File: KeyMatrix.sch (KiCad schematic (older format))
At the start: 100 parts, among them SW10 CherryMX, SW11 CherryMX, SW12 CherryMX, SW13 CherryMX, SW14 CherryMX, SW15 CherryMX, SW16 CherryMX, SW17 CherryMX, SW18 CherryMX, SW19 CherryMX, SW2 CherryMX, SW20 CherryMX, SW21 CherryMX, SW22 CherryMX, SW23 CherryMX, SW24 CherryMX, SW25 CherryMX, SW26 CherryMX, SW27 CherryMX, SW28 CherryMX, SW29 CherryMX, SW3 CherryMX, SW30 CherryMX, SW31 CherryMX, SW32 CherryMX, SW33 CherryMX, SW34 CherryMX, SW35 CherryMX, SW36 CherryMX, SW37 CherryMX, SW38 CherryMX, SW39 CherryMX, SW4 CherryMX, SW40 CherryMX, SW41 CherryMX, SW42 CherryMX, SW43 CherryMX, SW44 CherryMX, SW45 CherryMX, SW46 CherryMX, SW47 CherryMX, SW48 CherryMX, SW49 CherryMX, SW5 CherryMX, SW50 CherryMX, SW51 CherryMX, SW6 CherryMX, SW7 CherryMX, SW8 CherryMX, SW9 CherryMX

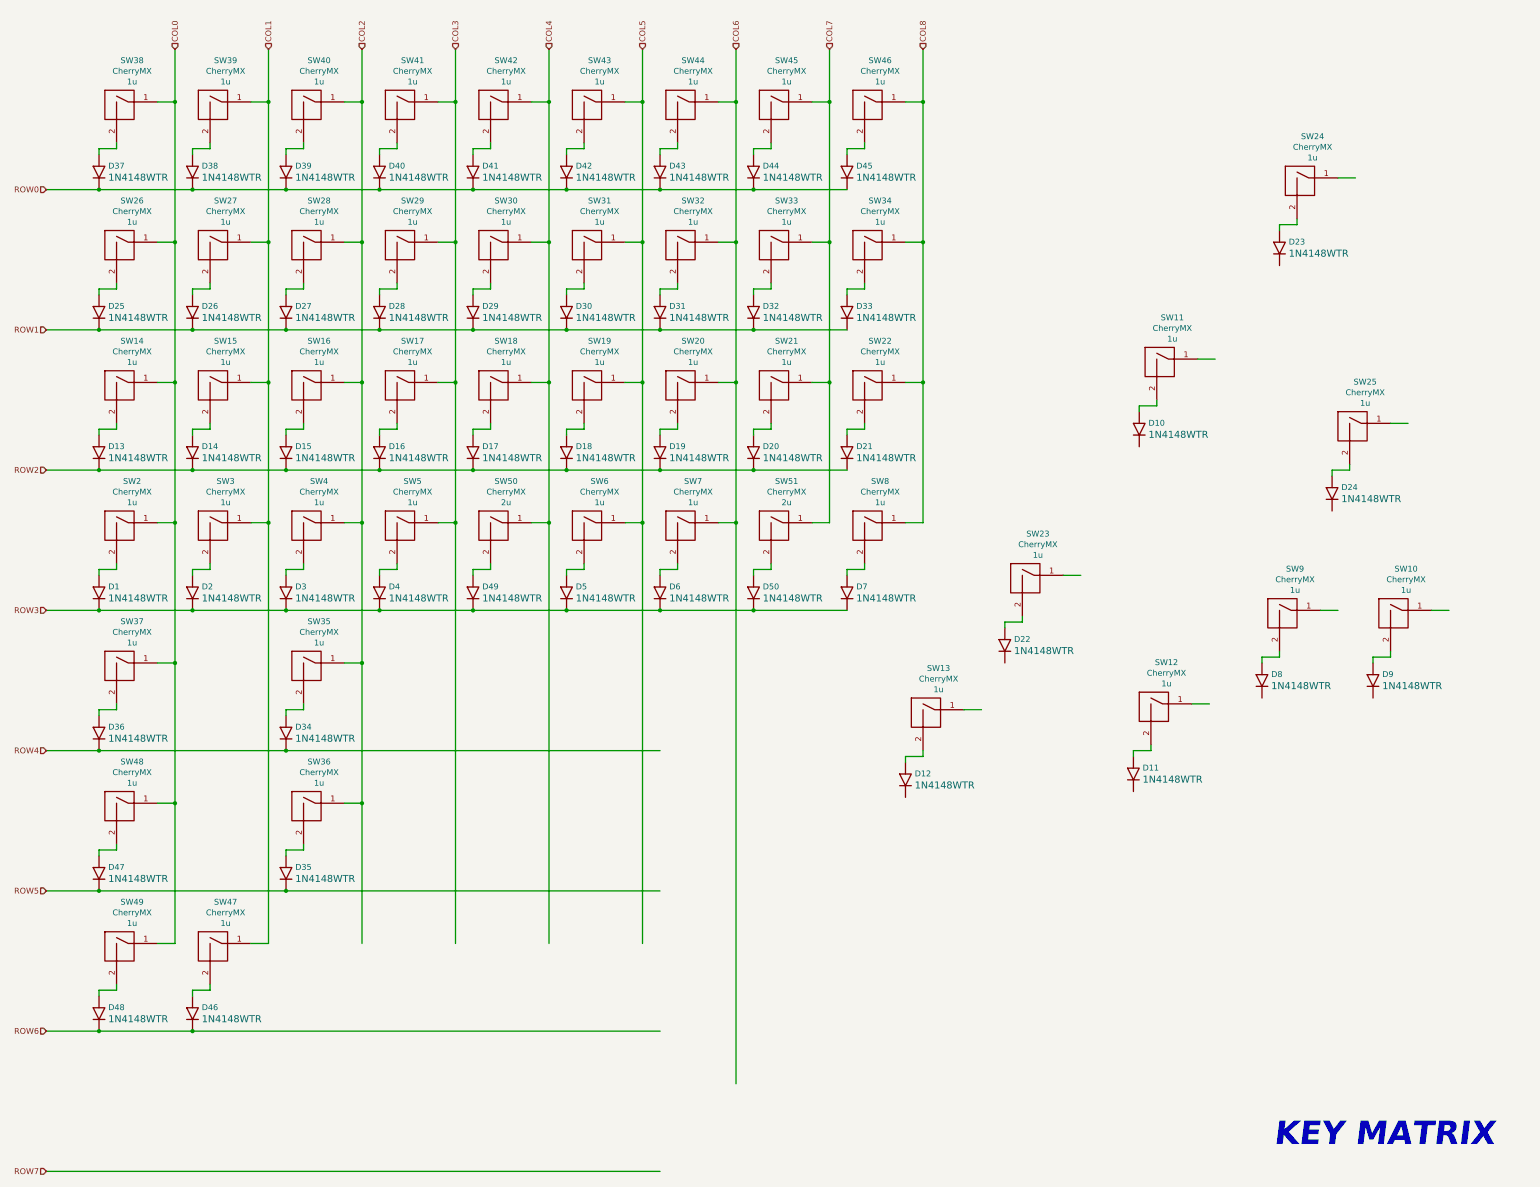
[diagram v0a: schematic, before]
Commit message: More Routing
more routing
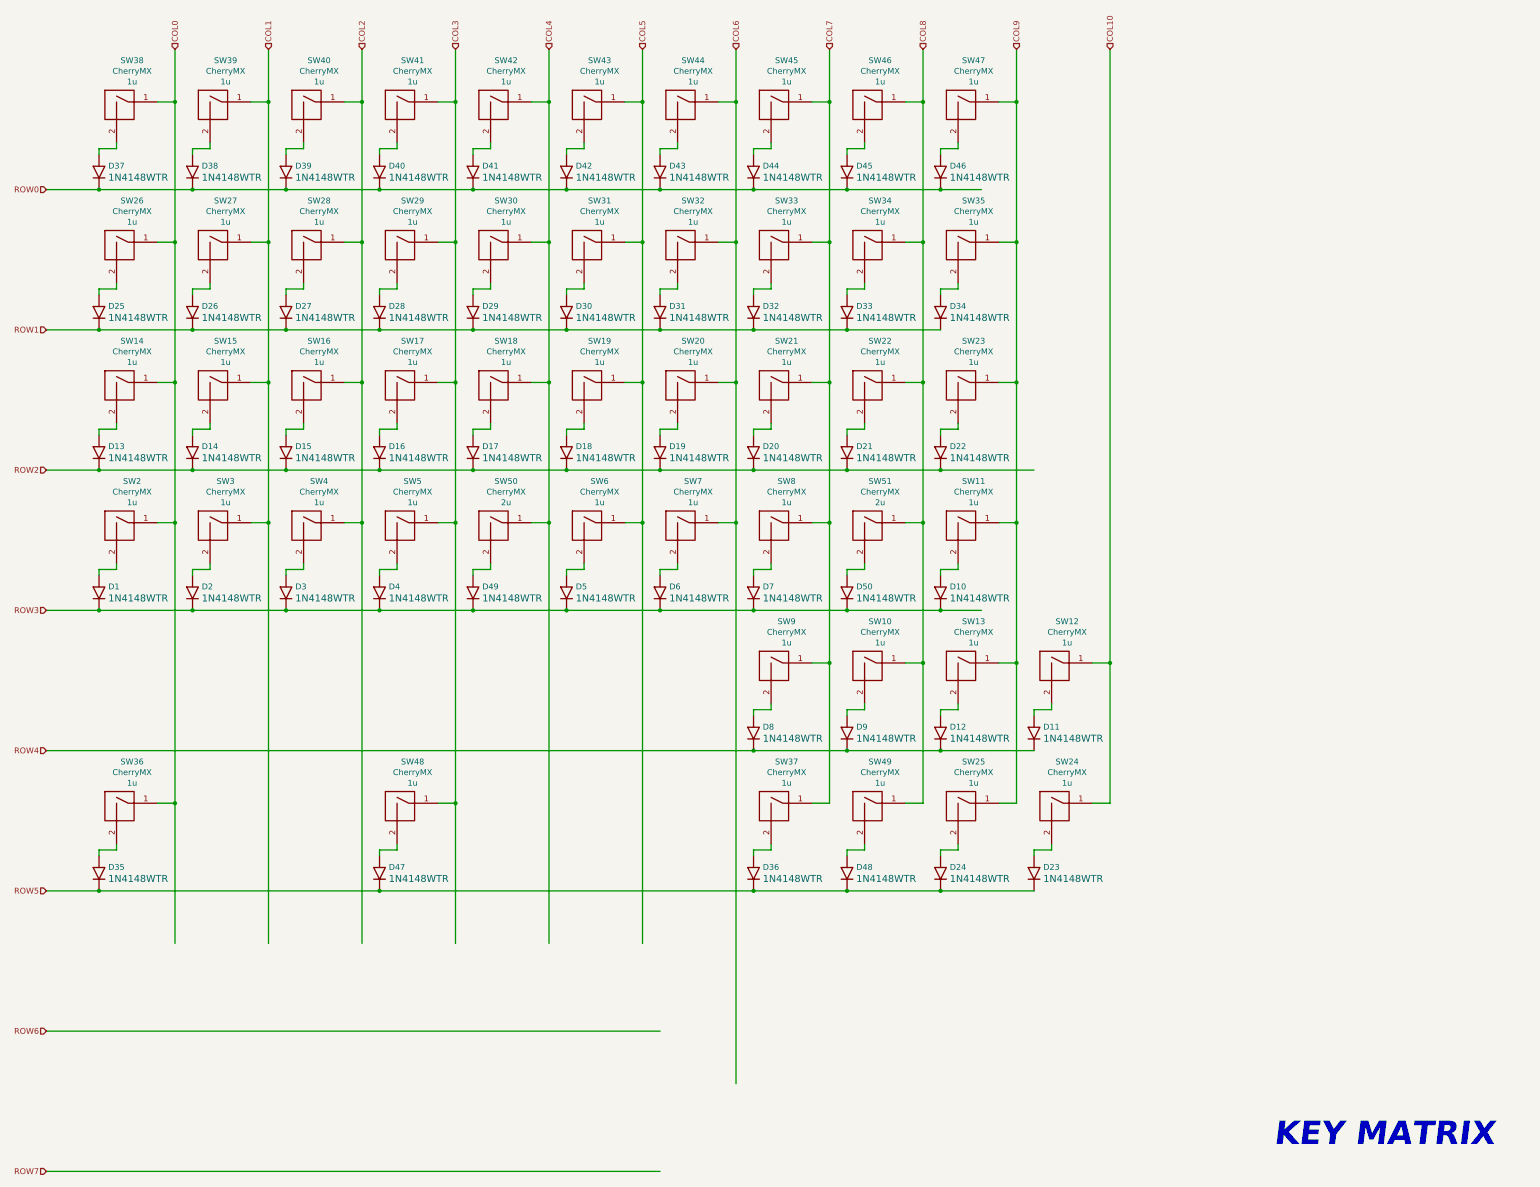
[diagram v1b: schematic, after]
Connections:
- net labels added: COL10, COL9
- wire segments 293 -> 312
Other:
- moved on the sheet: D10, D11, D12, D22, D23, D24, D34, D35, D36, D46, D47, D48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

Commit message: more routing
more routing
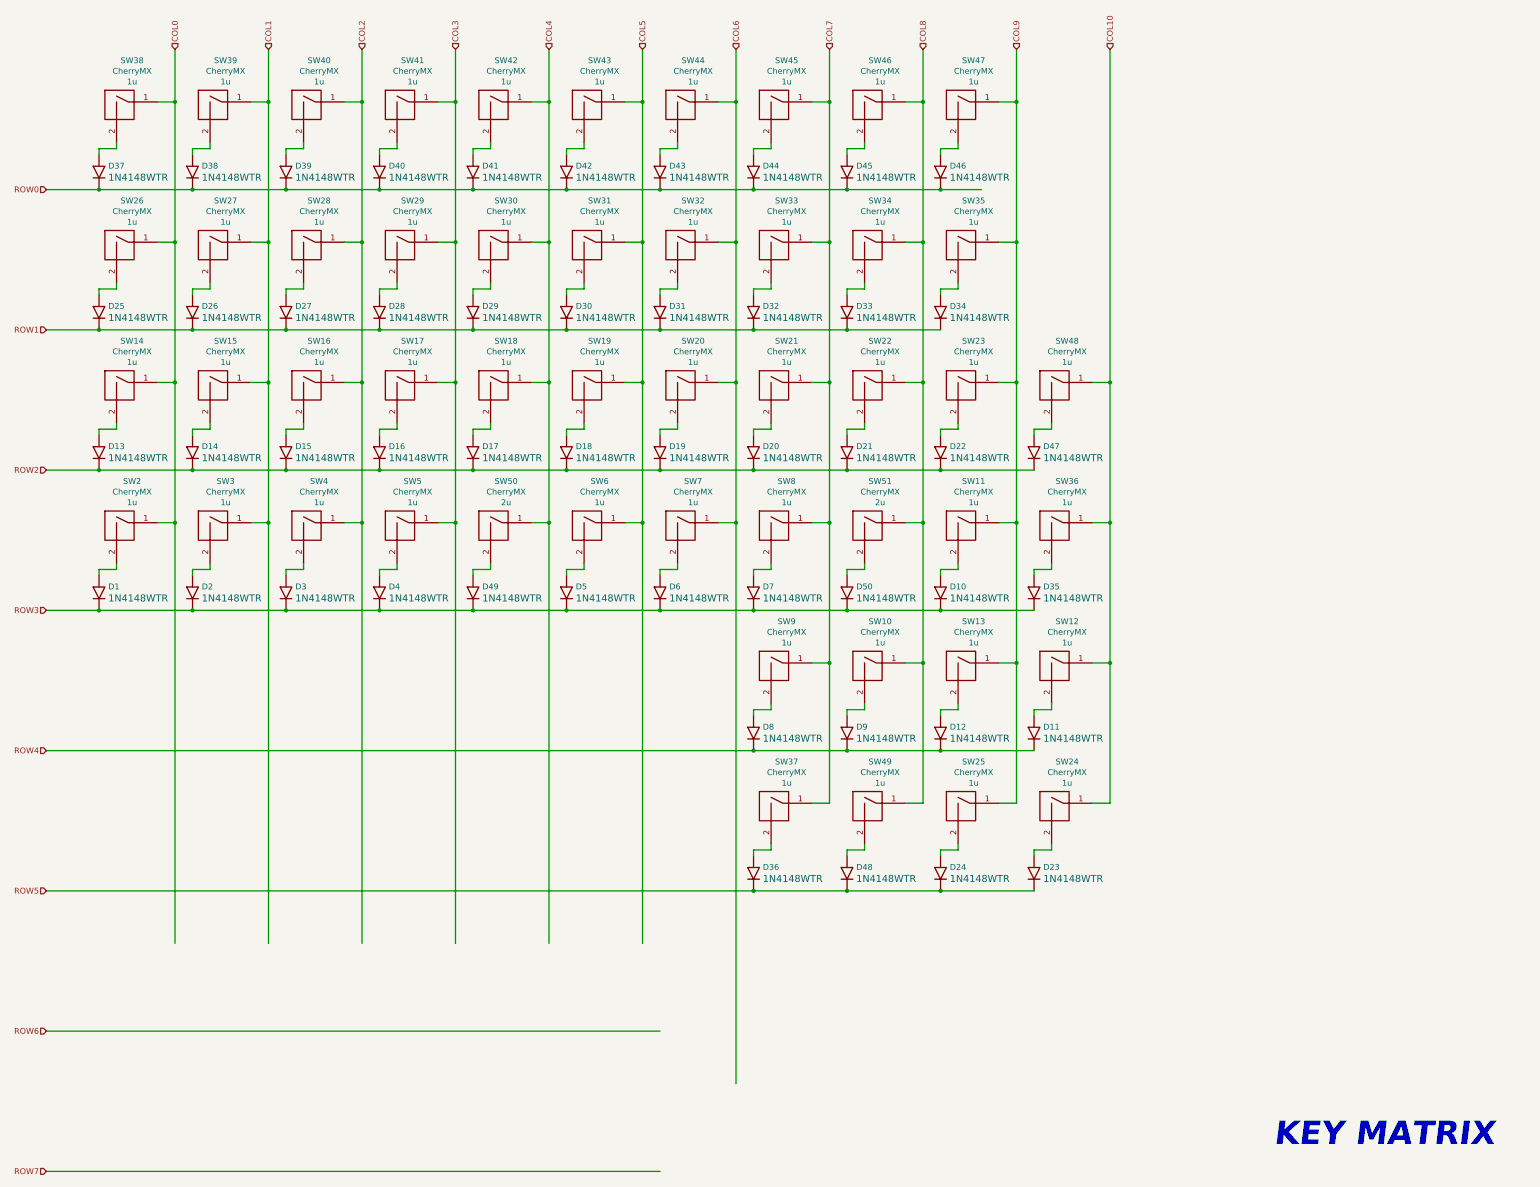
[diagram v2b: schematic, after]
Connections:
- wire segments 312 -> 310
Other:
- moved on the sheet: D35, D47, SW36, SW48
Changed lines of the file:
@@
 L MKB_Switches:CherryMX SW36
 U 1 1 5F4FA06B
-P 3000 7500
-F 0 "SW36" H 3133 7905 50  0000 C CNN
-F 1 "CherryMX" H 3133 7814 50  0000 C CNN
-F 2 "CherryMX:SW_Cherry-MX_1U_PCB-Mount_Kailh-Hot-Swap" H 3900 7600 50  0001 C CNN
-F 3 "" H 3800 7600 50  0001 C CNN
-F 4 "DNP" H 3000 7500 50  0001 C CNN "Manufacturer"
-F 5 "DNP" H 3000 7500 50  0001 C CNN "MPN"
-F 6 "DNP" H 3000 7500 50  0001 C CNN "Supplier"
-F 7 "DNP" H 3000 7500 50  0001 C CNN "Supplier PN"
-F 8 "1u" H 3133 7723 50  0000 C CNN "Package"
-	1    3000 7500
-	1    0    0    -1
-$EndComp
-Wire Wire Line
-	3500 7450 3350 7450
-Wire Wire Line
-	3000 7800 3000 7850
-Wire Wire Line
-	3000 7850 2850 7850
-Wire Wire Line
-	2850 7850 2850 7900
+P 11000 5100
+F 0 "SW36" H 11133 5505 50  0000 C CNN
+F 1 "CherryMX" H 11133 5414 50  0000 C CNN
+F 2 "CherryMX:SW_Cherry-MX_1U_PCB-Mount_Kailh-Hot-Swap" H 11900 5200 50  0001 C CNN
+F 3 "" H 11800 5200 50  0001 C CNN
+F 4 "DNP" H 11000 5100 50  0001 C CNN "Manufacturer"
+F 5 "DNP" H 11000 5100 50  0001 C CNN "MPN"
+F 6 "DNP" H 11000 5100 50  0001 C CNN "Supplier"
+F 7 "DNP" H 11000 5100 50  0001 C CNN "Supplier PN"
+F 8 "1u" H 11133 5323 50  0000 C CNN "Package"
+	1    11000 5100
+	1    0    0    -1
+$EndComp
+Wire Wire Line
+	11500 5050 11350 5050
+Wire Wire Line
+	11000 5400 11000 5450
+Wire Wire Line
+	11000 5450 10850 5450
+Wire Wire Line
+	10850 5450 10850 5500
 $Comp
 L master-vampire_General:D D35
 U 1 1 5F4FA080
-P 2850 8050
-F 0 "D35" V 2903 7971 50  0000 R CNN
-F 1 "D" H 3300 8250 50  0001 C CNN
-F 2 "ortho-40percent:SOD-123" H 2750 8050 50  0001 C CNN
-F 3 "" H 2850 8150 50  0001 C CNN
-F 4 "1N4148WTR" V 2804 7971 60  0000 R CNN "MPN"
-F 5 "SMC Diode Solutions" H 3300 8350 60  0001 C CNN "Manufacturer"
-F 6 "DigiKey" H 3150 8450 50  0001 C CNN "Supplier"
-F 7 "1655-1360-1-ND" H 3250 8550 50  0001 C CNN "Supplier PN"
-F 8 "75V" V 2850 7971 50  0001 R CNN "Voltage Rating"
-F 9 "250mA" V 2759 7971 50  0001 R CNN "Current Rating"
-F 10 "SOD-123" H 3550 8850 50  0001 C CNN "Package"
-	1    2850 8050
+P 10850 5650
+F 0 "D35" V 10903 5571 50  0000 R CNN
+F 1 "D" H 11300 5850 50  0001 C CNN
+F 2 "ortho-40percent:SOD-123" H 10750 5650 50  0001 C CNN
+F 3 "" H 10850 5750 50  0001 C CNN
+F 4 "1N4148WTR" V 10804 5571 60  0000 R CNN "MPN"
+F 5 "SMC Diode Solutions" H 11300 5950 60  0001 C CNN "Manufacturer"
+F 6 "DigiKey" H 11150 6050 50  0001 C CNN "Supplier"
+F 7 "1655-1360-1-ND" H 11250 6150 50  0001 C CNN "Supplier PN"
+F 8 "75V" V 10850 5571 50  0001 R CNN "Voltage Rating"
+F 9 "250mA" V 10759 5571 50  0001 R CNN "Current Rating"
+F 10 "SOD-123" H 11550 6450 50  0001 C CNN "Package"
+	1    10850 5650
 	0    -1   -1   0
 $EndComp
@@
 	6050 5800 6850 5800
 Connection ~ 6700 5050
-Wire Wire Line
-	2400 8200 2850 8200
-Connection ~ 2850 8200
-Connection ~ 3500 7450
-Wire Wire Line
-	3500 7450 3500 8650
 Connection ~ 9250 7000
 Connection ~ 8450 7000
 Wire Wire Line
 	8450 7000 9250 7000
-Wire Wire Line
-	3500 5050 3500 7450
 Wire Wire Line
 	9100 3850 9100 5050
@@
 Connection ~ 9900 6250
 Wire Wire Line
-	10050 5800 10400 5800
-Wire Wire Line
-	5250 8200 8450 8200
-Wire Wire Line
-	5900 5050 5900 7450
-Wire Wire Line
-	5900 7450 5900 8650
-Connection ~ 5900 7450
-Connection ~ 5250 8200
-Wire Wire Line
-	11500 1000 11500 6250
+	11500 1000 11500 3850
 $Comp
 L master-vampire_General:D D47
 U 1 1 5F4FA0C8
-P 5250 8050
-F 0 "D47" V 5303 7971 50  0000 R CNN
-F 1 "D" H 5700 8250 50  0001 C CNN
-F 2 "ortho-40percent:SOD-123" H 5150 8050 50  0001 C CNN
-F 3 "" H 5250 8150 50  0001 C CNN
-F 4 "1N4148WTR" V 5204 7971 60  0000 R CNN "MPN"
-F 5 "SMC Diode Solutions" H 5700 8350 60  0001 C CNN "Manufacturer"
-F 6 "DigiKey" H 5550 8450 50  0001 C CNN "Supplier"
-F 7 "1655-1360-1-ND" H 5650 8550 50  0001 C CNN "Supplier PN"
-F 8 "75V" V 5250 7971 50  0001 R CNN "Voltage Rating"
-F 9 "250mA" V 5159 7971 50  0001 R CNN "Current Rating"
-F 10 "SOD-123" H 5950 8850 50  0001 C CNN "Package"
-	1    5250 8050
-	0    -1   -1   0
-$EndComp
-Wire Wire Line
-	5250 7850 5250 7900
-Wire Wire Line
-	5400 7850 5250 7850
-Wire Wire Line
-	5400 7800 5400 7850
-Wire Wire Line
-	5900 7450 5750 7450
+P 10850 4450
+F 0 "D47" V 10903 4371 50  0000 R CNN
+F 1 "D" H 11300 4650 50  0001 C CNN
+F 2 "ortho-40percent:SOD-123" H 10750 4450 50  0001 C CNN
+F 3 "" H 10850 4550 50  0001 C CNN
+F 4 "1N4148WTR" V 10804 4371 60  0000 R CNN "MPN"
+F 5 "SMC Diode Solutions" H 11300 4750 60  0001 C CNN "Manufacturer"
+F 6 "DigiKey" H 11150 4850 50  0001 C CNN "Supplier"
+F 7 "1655-1360-1-ND" H 11250 4950 50  0001 C CNN "Supplier PN"
+F 8 "75V" V 10850 4371 50  0001 R CNN "Voltage Rating"
+F 9 "250mA" V 10759 4371 50  0001 R CNN "Current Rating"
+F 10 "SOD-123" H 11550 5250 50  0001 C CNN "Package"
+	1    10850 4450
+	0    -1   -1   0
+$EndComp
+Wire Wire Line
+	10850 4250 10850 4300
+Wire Wire Line
+	11000 4250 10850 4250
+Wire Wire Line
+	11000 4200 11000 4250
+Wire Wire Line
+	11500 3850 11350 3850
 $Comp
 L MKB_Switches:CherryMX SW48
 U 1 1 5F4FA0B3
-P 5400 7500
-F 0 "SW48" H 5533 7905 50  0000 C CNN
-F 1 "CherryMX" H 5533 7814 50  0000 C CNN
-F 2 "CherryMX:SW_Cherry-MX_1U_PCB-Mount_Kailh-Hot-Swap" H 6300 7600 50  0001 C CNN
-F 3 "" H 6200 7600 50  0001 C CNN
-F 4 "DNP" H 5400 7500 50  0001 C CNN "Manufacturer"
-F 5 "DNP" H 5400 7500 50  0001 C CNN "MPN"
-F 6 "DNP" H 5400 7500 50  0001 C CNN "Supplier"
-F 7 "DNP" H 5400 7500 50  0001 C CNN "Supplier PN"
-F 8 "1u" H 5533 7723 50  0000 C CNN "Package"
-	1    5400 7500
+P 11000 3900
+F 0 "SW48" H 11133 4305 50  0000 C CNN
+F 1 "CherryMX" H 11133 4214 50  0000 C CNN
+F 2 "CherryMX:SW_Cherry-MX_1U_PCB-Mount_Kailh-Hot-Swap" H 11900 4000 50  0001 C CNN
+F 3 "" H 11800 4000 50  0001 C CNN
+F 4 "DNP" H 11000 3900 50  0001 C CNN "Manufacturer"
+F 5 "DNP" H 11000 3900 50  0001 C CNN "MPN"
+F 6 "DNP" H 11000 3900 50  0001 C CNN "Supplier"
+F 7 "DNP" H 11000 3900 50  0001 C CNN "Supplier PN"
+F 8 "1u" H 11133 4123 50  0000 C CNN "Package"
+	1    11000 3900
 	1    0    0    -1
 $EndComp
@@
 Wire Wire Line
 	4300 5050 4300 8650
-Wire Wire Line
-	2850 8200 5250 8200
+Connection ~ 11500 5050
+Wire Wire Line
+	11500 5050 11500 6250
+Wire Wire Line
+	3500 5050 3500 8650
+Wire Wire Line
+	10050 5800 10850 5800
+Connection ~ 11500 3850
+Wire Wire Line
+	11500 3850 11500 5050
+Wire Wire Line
+	2400 8200 8450 8200
+Wire Wire Line
+	5900 5050 5900 8650
 $EndSCHEMATC
